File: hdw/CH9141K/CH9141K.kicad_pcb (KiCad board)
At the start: 2 copper layers, 34.3 x 19.3 mm, 6 parts, among them J1 Conn_01x04, U1 CH9141K, Y1 32M

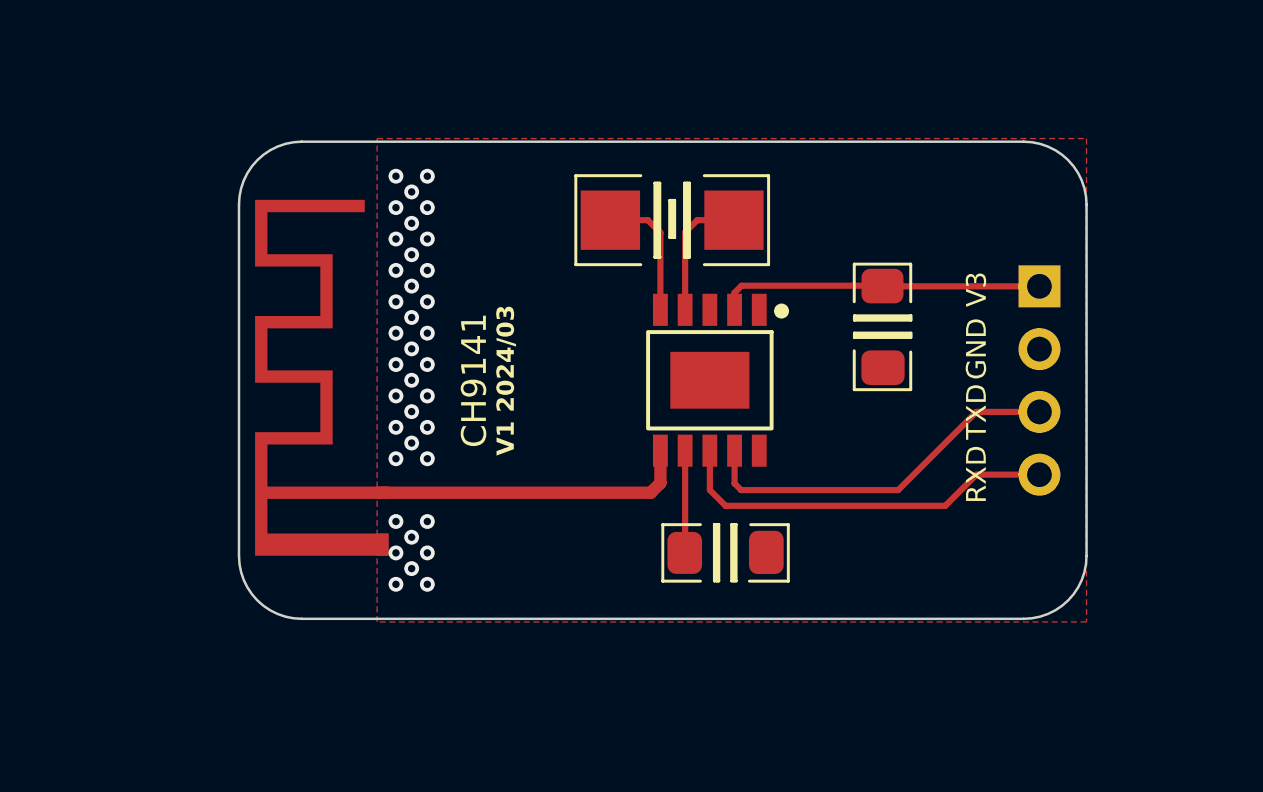
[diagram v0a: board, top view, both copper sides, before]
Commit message: wip
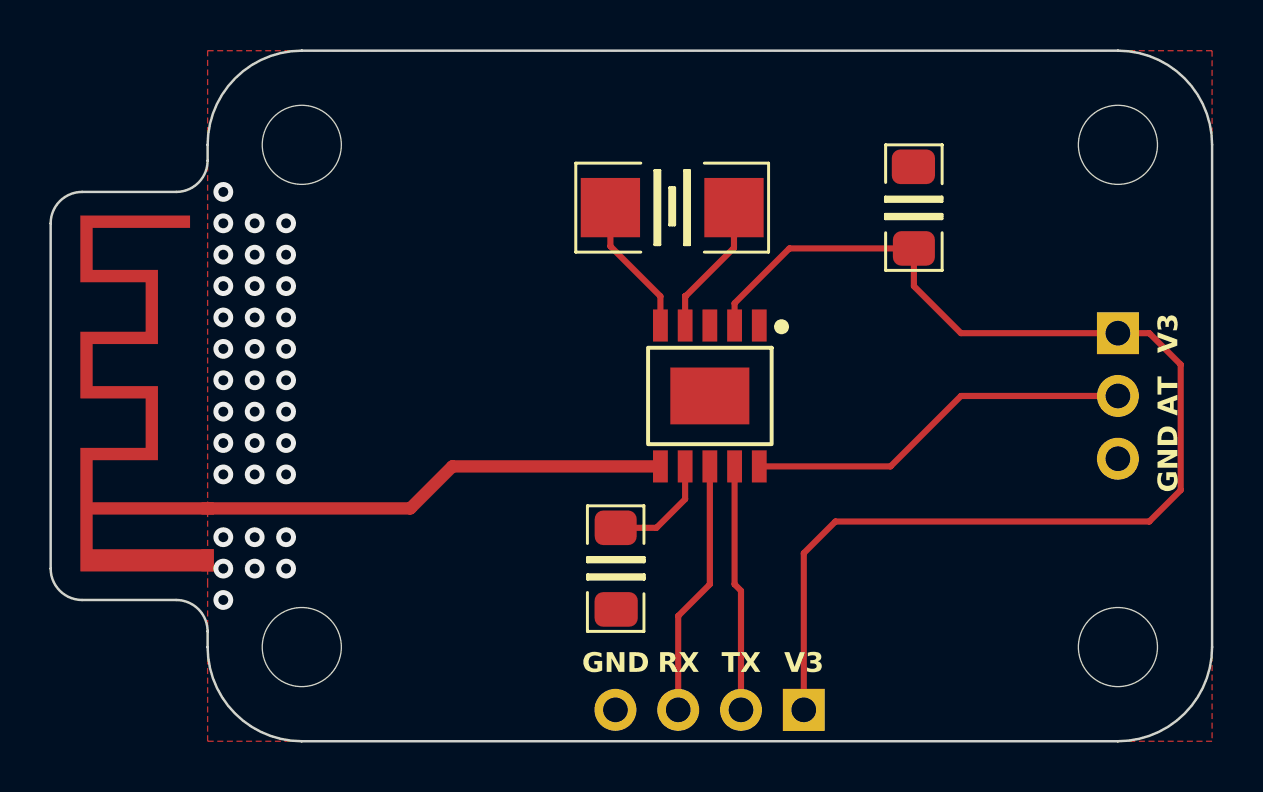
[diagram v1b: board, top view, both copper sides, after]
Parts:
- removed AE1: Antenna, RF_Antenna:Texas_SWRA117D_2.4GHz_Right
- removed J1: Conn_01x04, Connector_PinHeader_2.54mm:PinHeader_1x04_P2.54mm_Vertical
- added AE2: Antenna_Shield, RF_Antenna:Texas_SWRA117D_2.4GHz_Right, F.Cu at (72.4, 118.8)
- added H1: MountingHole, MountingHole:MountingHole_3.2mm_M3, F.Cu at (76.2, 104.1)
- added H2: MountingHole, MountingHole:MountingHole_3.2mm_M3, F.Cu at (109.2, 104.1)
- added H3: MountingHole, MountingHole:MountingHole_3.2mm_M3, F.Cu at (109.2, 124.5)
- added H4: MountingHole, MountingHole:MountingHole_3.2mm_M3, F.Cu at (76.2, 124.5)
- added J2: Conn_01x03, Connector_PinHeader_2.54mm:PinHeader_1x03_P2.54mm_Vertical, F.Cu at (109.2, 111.8)
- added J3: Conn_01x04, Connector_PinHeader_2.54mm:PinHeader_1x04_P2.54mm_Vertical, F.Cu at (96.5, 127.0)
- moved C1 4.99 mm to (101.0, 106.7), turned to 90 degrees
- moved C2 4.49 mm to (88.9, 121.3), turned to -90 degrees
- moved U1 0.63 mm to (92.7, 114.3)
- moved Y1 0.51 mm to (91.2, 106.7)
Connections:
- U1 pad 10: GND -> AT
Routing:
- net VCC: track 13.2 -> 50.4 mm
- net AT: track 0.00 -> 15.7 mm
- net Net-(AE2-A): track 12.7 -> 19.0 mm
- net RXD: track 15.7 -> 10.4 mm
- net TXD: track 15.1 -> 9.96 mm
- net GND: vias 37 -> 35
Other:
- board size 34.3 x 19.3 mm -> 47 x 27.9 mm
- board text added: "AT"
- board text added: "CH9141K"
- board text added: "RX"
- board text added: "TX"
- board text added: "V1.1 2024-04"
- board text added: "nicola@strappazzon.me"
- board text removed: "CH9141"
- board text removed: "RXD"
- board text removed: "TXD"
- board text removed: "V1 2024/03"
- board text removed: "nstrappazzonc"
